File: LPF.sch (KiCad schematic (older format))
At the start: 125 parts, among them J1 Conn_02x05_Counter_Clockwise, P1 SMA, P3 SMA, P4 SMA

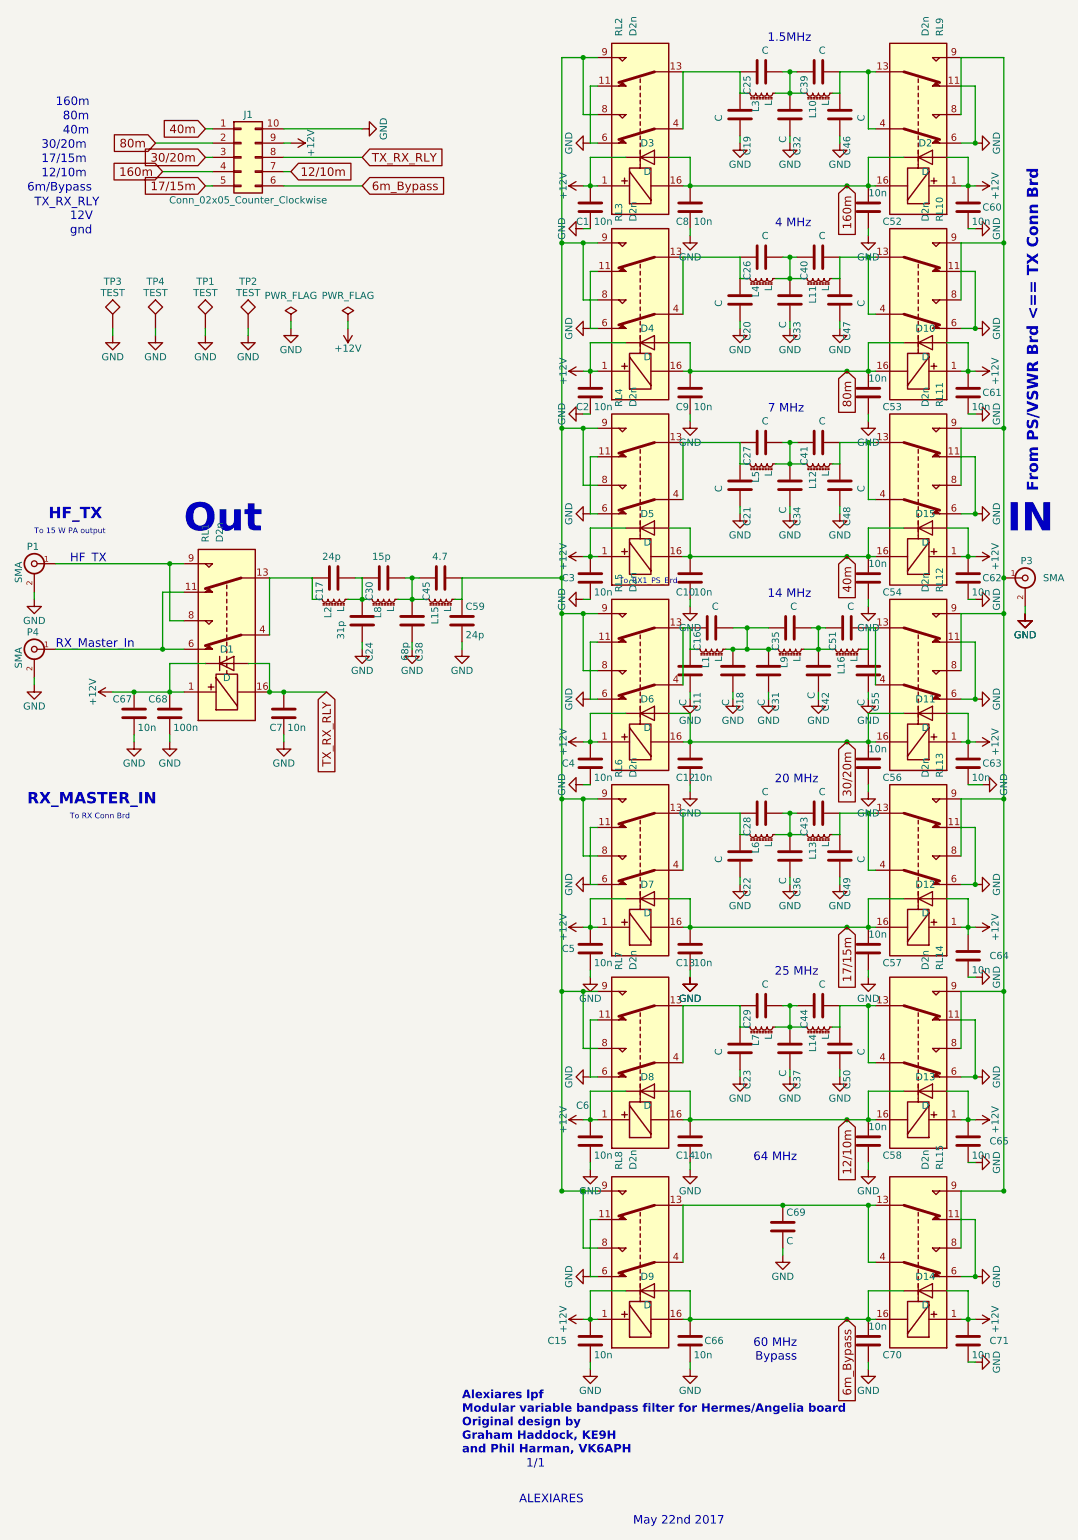
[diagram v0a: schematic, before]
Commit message: RTM
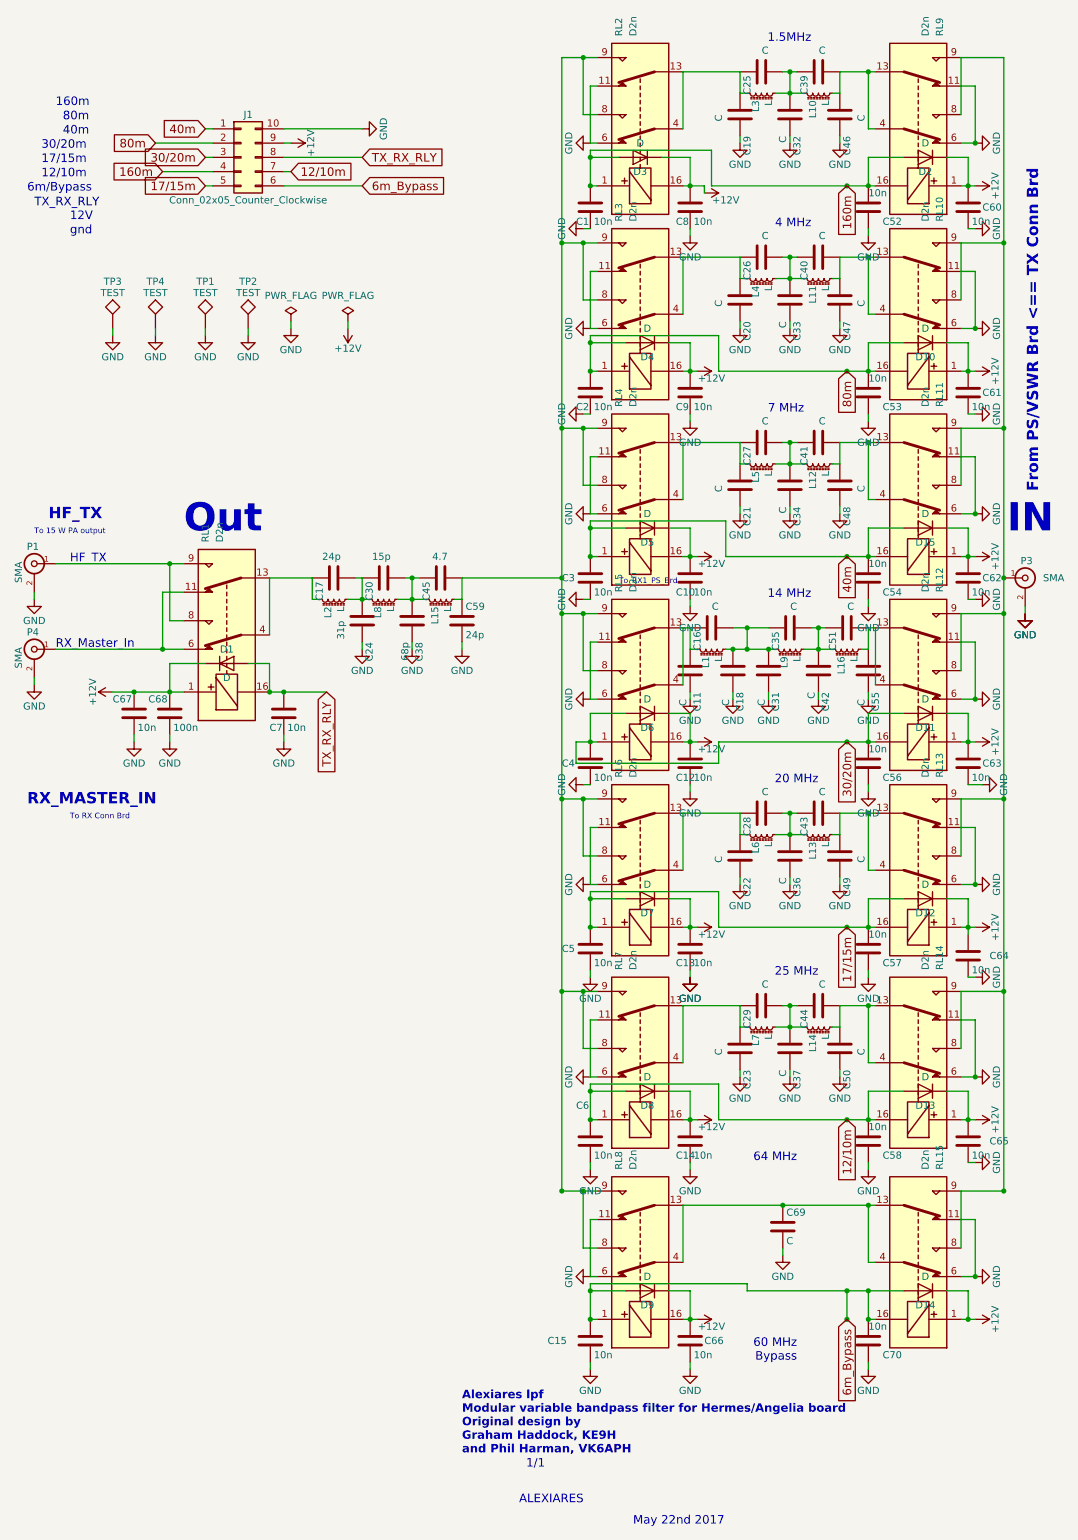
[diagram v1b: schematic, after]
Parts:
- removed C71: 10n, Capacitors_SMD:C_0805_HandSoldering, symbol C
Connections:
- net +12V: now also C10.1, C12.1, C13.1, C14.1, C66.1, C8.1, C9.1, D10.1 (K), D11.1 (K), D12.1 (K), D13.1 (K), D14.1 (K), D15.1 (K), D2.1 (K), RL2.16, RL3.16, RL4.16, RL5.16, RL6.16, RL7.16, RL8.16; no longer C1.1, C15.1, C2.1, C3.1, C4.1, C5.1, C6.1, D10.2 (A), D11.2 (A), D12.2 (A), D13.2 (A), D14.2 (A), D15.2 (A), D2.2 (A), RL2.1, RL3.1, RL4.1, RL5.1, RL6.1, RL7.1, RL8.1
- net 12/10m: now also C6.1, D13.2 (A), RL7.1; no longer C14.1, D13.1 (K), RL7.16
- net 160m: now also C1.1, D2.2 (A), RL2.1; no longer C8.1, D2.1 (K), RL2.16
- net 17/15m: now also C5.1, D12.2 (A), RL6.1; no longer C13.1, D12.1 (K), RL6.16
- net 30/20m: now also C4.1, D11.2 (A), RL5.1; no longer C12.1, D11.1 (K), RL5.16
- net 40m: now also C3.1, D15.2 (A), RL4.1; no longer C10.1, D15.1 (K), RL4.16
- net 6m_Bypass: now also C15.1, D14.2 (A), RL8.1; no longer C66.1, D14.1 (K), RL8.16
- net 80m: now also C2.1, D10.2 (A), RL3.1; no longer C9.1, D10.1 (K), RL3.16
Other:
- moved on the sheet: D3
